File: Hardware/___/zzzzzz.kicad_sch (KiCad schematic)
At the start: 8 parts, among them J1 Conn_01x07_Male, J2 Conn_01x04_Male, J3 Conn_01x02_Male, J4 Conn_01x02_Male, J5 Conn_01x02_Male, J6 Conn_01x02_Male, J7 Conn_01x08_Male, J9 QWIIC_Stackable

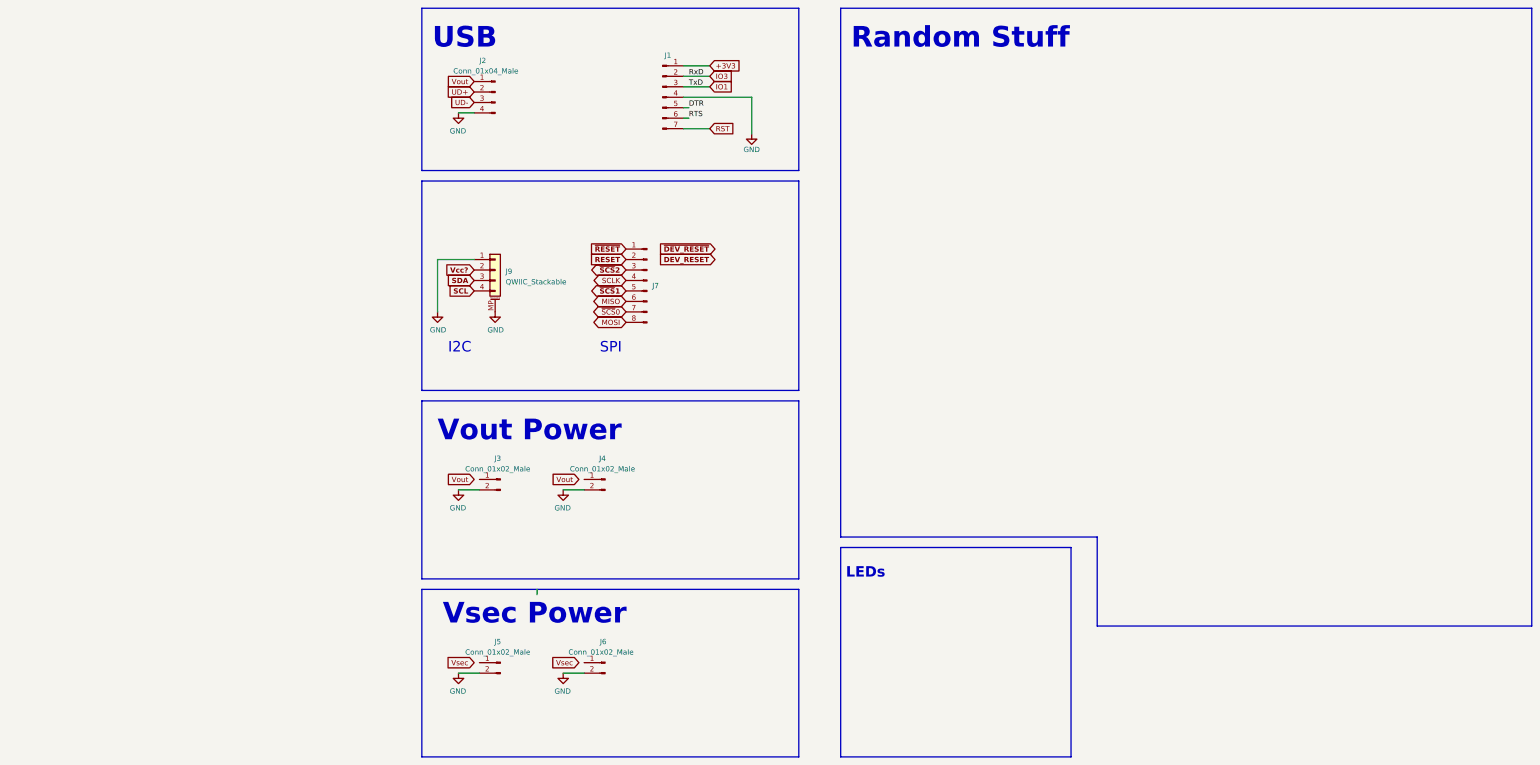
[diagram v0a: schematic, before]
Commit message: Working on the RP2040 & cleaning up stuff...
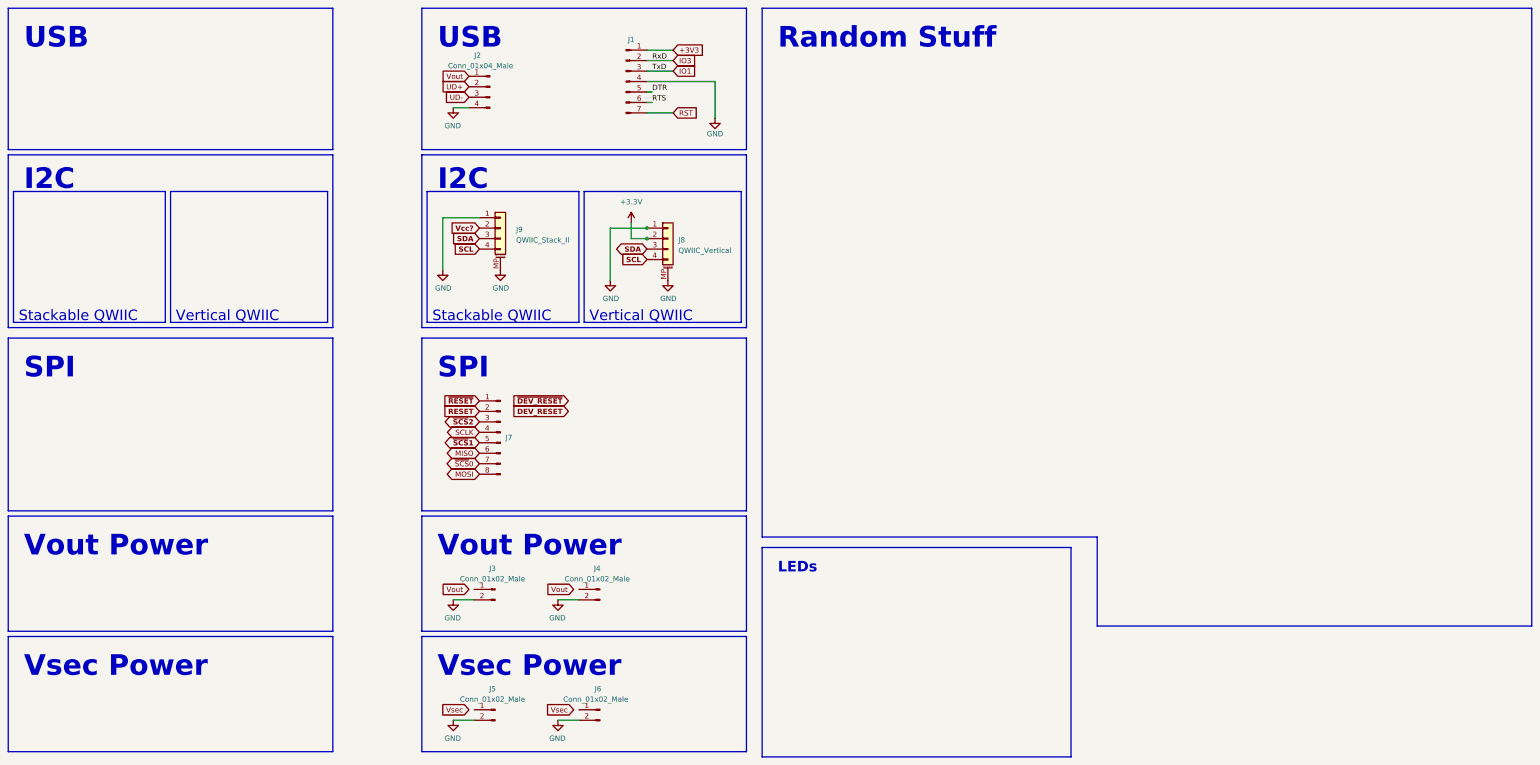
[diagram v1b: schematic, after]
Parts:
- added J8: QWIIC_Vertical, Tinker:QWIIC_Vertical, symbol Connector_Generic_MountingPin:Conn_01x04_MountingPin
- J9: value QWIIC_Stackable -> QWIIC_Stack_II
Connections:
- net +3V3: now also J8.2 (Pin_2)
- net GND: now also J8.1 (Pin_1), J8.MP (MountPin)
- net SCL: now also J8.4 (Pin_4)
- net SDA: now also J8.3 (Pin_3)
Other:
- note added: "Stackable QWIIC"
- note added: "Vertical QWIIC"
- moved on the sheet: J1, J2, J3, J4, J5, J6, J7, J9
